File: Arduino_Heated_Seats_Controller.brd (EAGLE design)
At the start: 32.7 x 38.1 mm, 24 parts, among them U1 MEGA8-AI, U2 UA78M05CDCY, U3 ULN2003ADE4, U4 IC_TD62783-SO-18W

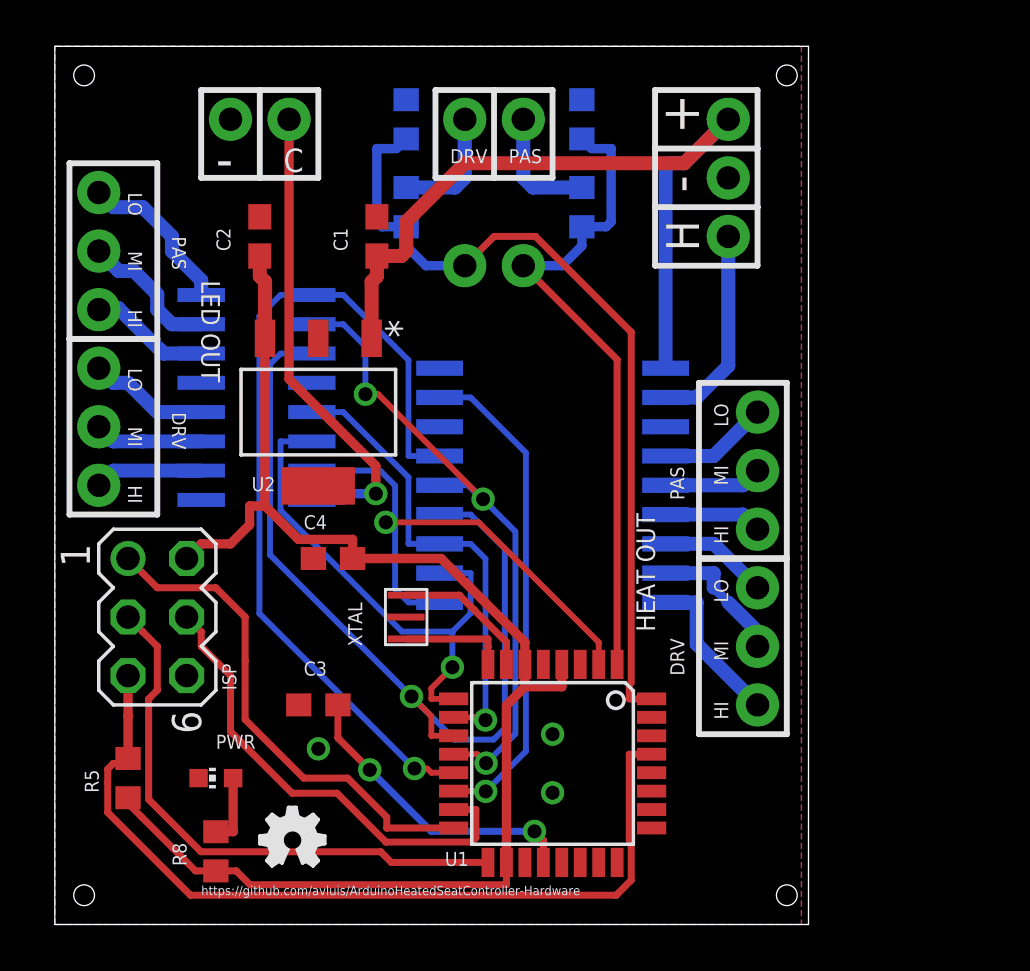
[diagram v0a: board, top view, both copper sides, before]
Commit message: Changes so far - commit before tweaking trace width and misc.
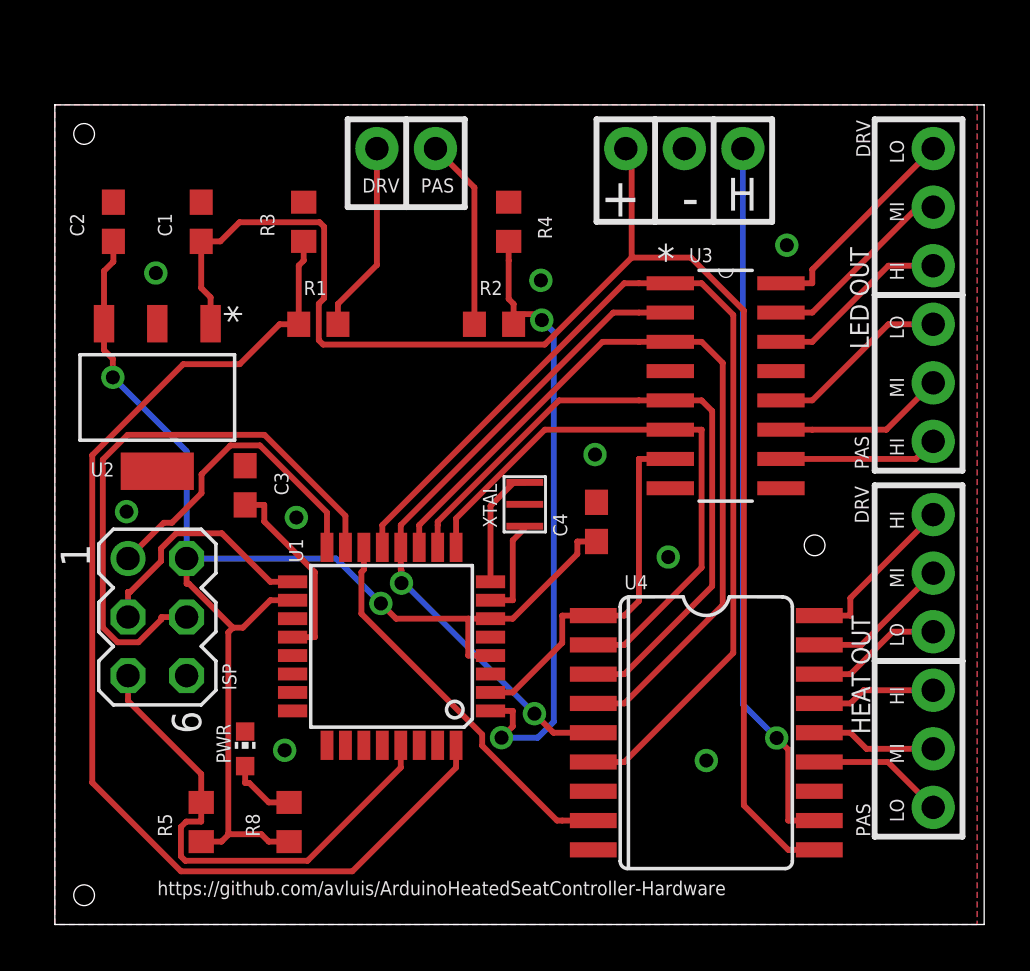
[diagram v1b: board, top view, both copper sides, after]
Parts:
- removed BTN-TEST, LED-TEST: (no value), SparkFun-Connectors:1X02
- U$1: device Logo:OSHW_FILLX100_NOTEXT -> Logo:OSHW_10X500_NOTEXT
- moved LED-OUT 36.2 mm to (38.1, 21.0)
- moved U3 25.2 mm to (31.5, 18.9), flipped to the top
- moved U$1 20.6 mm to (26.0, 14.0), flipped to the bottom
- moved U4 11.6 mm to (28.3, 8.95), flipped to the top, turned to 270 degrees
- moved C4 11.5 mm to (23.5, 17.5), turned to 90 degrees
- moved H-OUT 11.2 mm to (38.1, 17.8), turned to 270 degrees
- moved C3 10.0 mm to (8.26, 19.1), turned to 90 degrees
- moved U1 8.64 mm to (14.6, 12.1), turned to 180 degrees
- moved C1 7.65 mm to (6.35, 30.5)
- moved XTAL 7.10 mm to (20.4, 18.2), turned to 90 degrees
- moved U2 7.01 mm to (4.45, 22.9)
- moved C2 6.38 mm to (2.54, 30.5)
- moved R1 6.35 mm to (11.4, 26.0), flipped to the top, turned to 180 degrees
- moved R2 6.35 mm to (19.1, 26.0), flipped to the top, turned to 0 degrees
- moved R3 6.29 mm to (10.8, 30.5), flipped to the top
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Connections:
- removed net L-TEST: LED-TEST.1, U3.8
- net D2: no longer BTN-TEST.1
- net D3: no longer BTN-TEST.2
- net GND: now also U3.8; no longer LED-TEST.2, U3.9
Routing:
- net VIN: track 34.4 -> 65.9 mm
- net H-ON: track 8.90 -> 31.3 mm, vias 0 -> 1
- net L-TEST: track 20.7 -> 0.00 mm, vias 1 -> 0
- net RESET: track 37.5 -> 22.2 mm
- net D13: track 24.4 -> 10.5 mm
- net D2: track 36.1 -> 49.4 mm
- net D6: track 20.3 -> 29.7 mm, vias 1 -> 0
- net D12: track 21.8 -> 13.9 mm
- net D4: track 23.3 -> 16.3 mm, vias 1 -> 0
- net D9: track 37.7 -> 43.8 mm, vias 1 -> 0
- net D11: track 20.6 -> 25.5 mm
- net AREF: track 13.1 -> 8.44 mm, vias 2 -> 0
- net D10: track 21.5 -> 17.0 mm, vias 1 -> 0
- net D5: track 22.4 -> 25.6 mm, vias 1 -> 0
- net D-BTN: track 5.25 -> 8.32 mm
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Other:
- board size 32.7 x 38.1 mm -> 40.3 x 35.5 mm
- board text added: "Arduino Powered Heated Seat Controller rev. 4"
- board text removed: "Arduino Powered Heated Seat Controller rev. 3"
- board text removed: "C"
